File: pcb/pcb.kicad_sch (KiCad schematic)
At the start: 20 parts, among them J1 Conn_01x03_Pin, J2 Screw_Terminal_01x06, J3 Barrel_Jack_Switch, J5 DE9_Plug, U1 74LS165, U2 LM7805_TO220

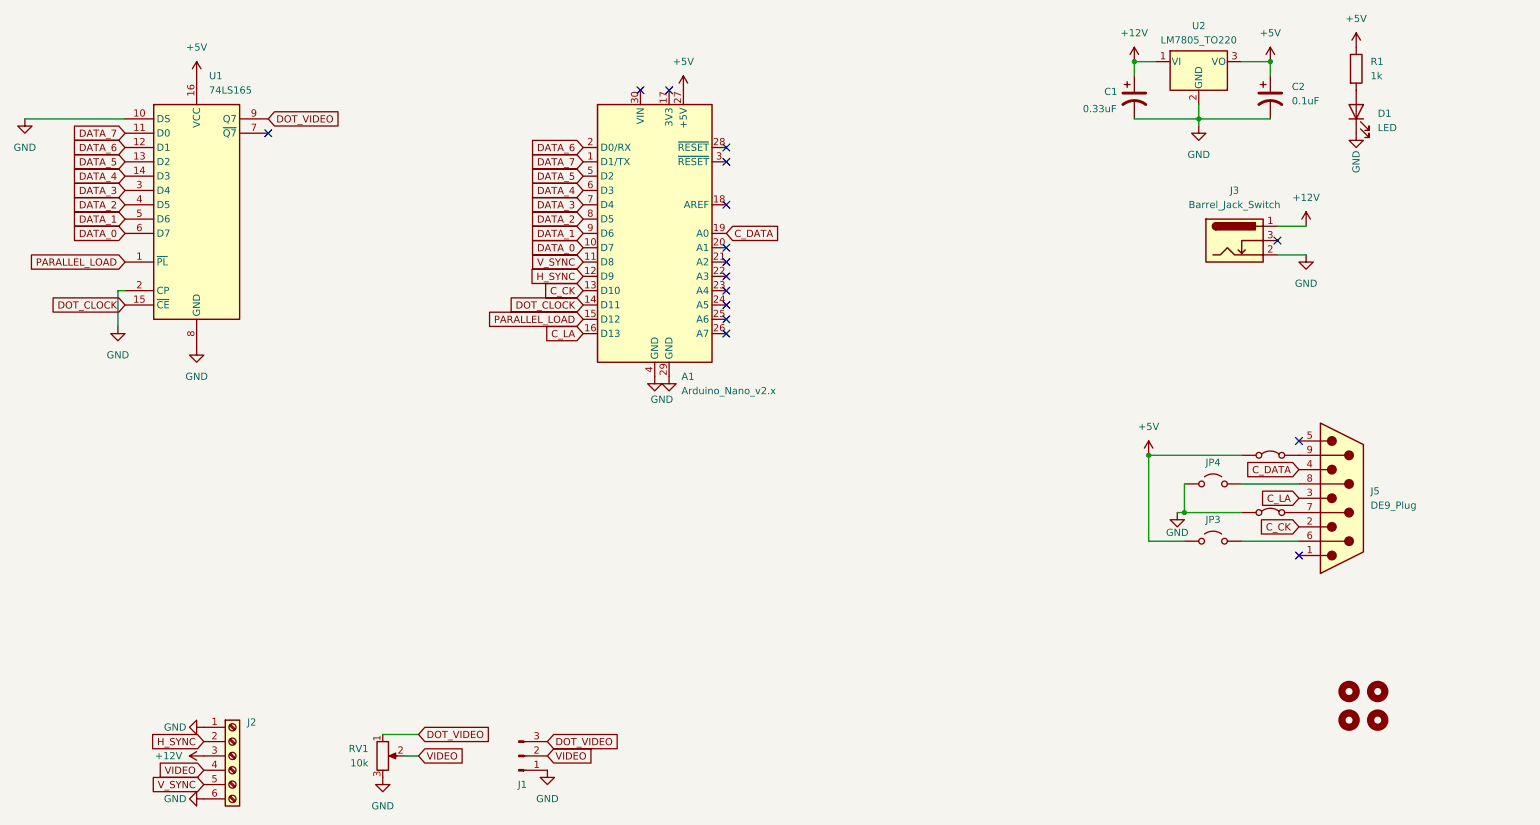
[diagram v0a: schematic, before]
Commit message: New PDB files
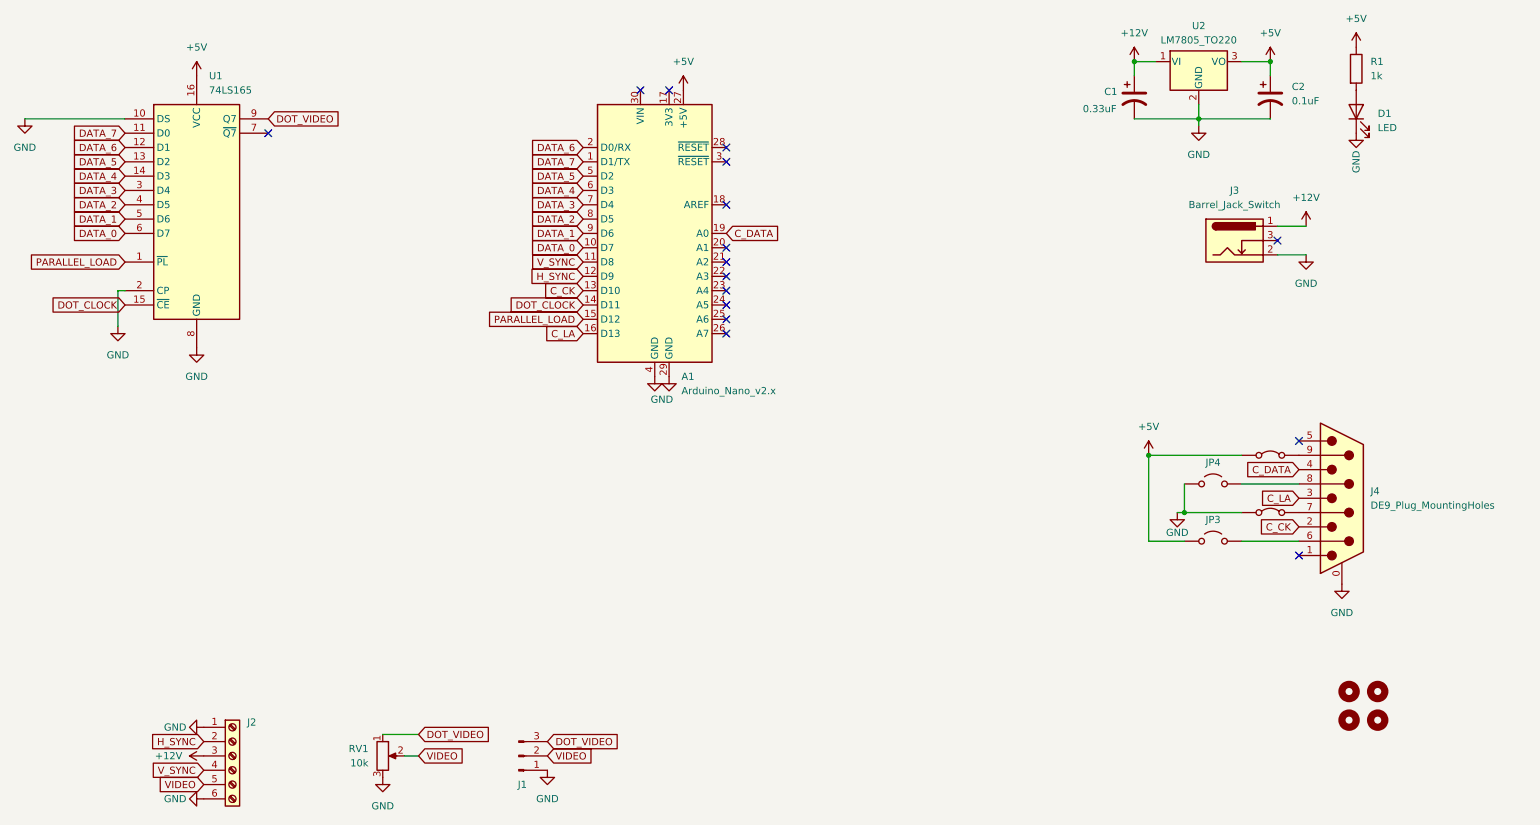
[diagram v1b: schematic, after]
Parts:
- removed J5: DE9_Plug, Connector_Dsub:DSUB-9_Female_Horizontal_P2.77x2.84mm_EdgePinOffset7.70mm_Housed_MountingHolesOffset9.12mm, symbol Connector:DE9_Plug
- added J4: DE9_Plug_MountingHoles, Connector_Dsub:DSUB-9_Female_Horizontal_P2.77x2.84mm_EdgePinOffset7.70mm_Housed_MountingHolesOffset9.12mm, symbol Connector:DE9_Plug_MountingHoles
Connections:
- net C_CK: now also J4.2
- net C_DATA: now also J4.4
- net C_LA: now also J4.3
- net GND: now also J4.0 (PAD)
- net VIDEO: now also J2.5 (Pin_5); no longer J2.4 (Pin_4)
- net V_SYNC: now also J2.4 (Pin_4); no longer J2.5 (Pin_5)
- net at JP3.2 (B): now also J4.6
- net at JP2.2 (B): now also J4.7
- net at JP4.2 (B): now also J4.8
- net at JP1.2 (B): now also J4.9
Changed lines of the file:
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@@
 	(global_label "V_SYNC"
 		(shape input)
-		(at 60.96 161.29 180)
+		(at 60.96 158.75 180)
 		(fields_autoplaced yes)
 		(effects
@@
 		)
 		(property "Intersheetrefs" "${INTERSHEET_REFS}"
-			(at 51.02 161.29 0)
+			(at 51.02 158.75 0)
 			(effects
 				(font
@@
 	(global_label "VIDEO"
 		(shape input)
-		(at 60.96 158.75 180)
+		(at 60.96 161.29 180)
 		(fields_autoplaced yes)
 		(effects
@@
 		)
 		(property "Intersheetrefs" "${INTERSHEET_REFS}"
-			(at 52.5319 158.75 0)
+			(at 52.5319 161.29 0)
 			(effects
 				(font
@@
 	)
 	(symbol
-		(lib_id "Connector:DE9_Plug")
-		(at 262.89 110.49 0)
-		(unit 1)
-		(exclude_from_sim no)
-		(in_bom yes)
-		(on_board yes)
-		(dnp no)
-		(fields_autoplaced yes)
-		(property "Reference" "J5"
-			(at 267.97 109.2199 0)
-			(effects
-				(font
-					(size 1.27 1.27)
-				)
-				(justify left)
-			)
-		)
-		(property "Value" "DE9_Plug"
-			(at 267.97 111.7599 0)
-			(effects
-				(font
-					(size 1.27 1.27)
-				)
-				(justify left)
-			)
-		)
-		(property "Footprint" "Connector_Dsub:DSUB-9_Female_Horizontal_P2.77x2.84mm_EdgePinOffset7.70mm_Housed_MountingHolesOffset9.12mm"
-			(at 262.89 110.49 0)
-			(effects
-				(font
-					(size 1.27 1.27)
-				)
-				(hide yes)
-			)
-		)
-		(property "Datasheet" "~"
-			(at 262.89 110.49 0)
-			(effects
-				(font
-					(size 1.27 1.27)
-				)
-				(hide yes)
-			)
-		)
-		(property "Description" "9-pin male plug pin D-SUB connector"
-			(at 262.89 110.49 0)
-			(effects
-				(font
-					(size 1.27 1.27)
-				)
-				(hide yes)
-			)
-		)
-		(pin "8"
-		)
-		(pin "9"
-		)
-		(pin "1"
-		)
-		(pin "3"
-		)
-		(pin "5"
-		)
-		(pin "7"
-		)
-		(pin "2"
-		)
-		(pin "4"
-		)
-		(pin "6"
-		)
-		(instances
-			(project ""
-				(path "/e222e52e-83a8-4556-a94e-a22482ba41c4"
-					(reference "J5")
-					(unit 1)
-				)
-			)
-		)
-	)
-	(symbol
 		(lib_id "power:GND")
 		(at 233.68 113.03 0)
@@
 	)
 	(symbol
+		(lib_id "Connector:DE9_Plug_MountingHoles")
+		(at 262.89 110.49 0)
+		(unit 1)
+		(exclude_from_sim no)
+		(in_bom yes)
+		(on_board yes)
+		(dnp no)
+		(fields_autoplaced yes)
+		(property "Reference" "J4"
+			(at 267.97 109.2199 0)
+			(effects
+				(font
+					(size 1.27 1.27)
+				)
+				(justify left)
+			)
+		)
+		(property "Value" "DE9_Plug_MountingHoles"
+			(at 267.97 111.7599 0)
+			(effects
+				(font
+					(size 1.27 1.27)
+				)
+				(justify left)
+			)
+		)
+		(property "Footprint" "Connector_Dsub:DSUB-9_Female_Horizontal_P2.77x2.84mm_EdgePinOffset7.70mm_Housed_MountingHolesOffset9.12mm"
+			(at 262.89 110.49 0)
+			(effects
+				(font
+					(size 1.27 1.27)
+				)
+				(hide yes)
+			)
+		)
+		(property "Datasheet" "~"
+			(at 262.89 110.49 0)
+			(effects
+				(font
+					(size 1.27 1.27)
+				)
+				(hide yes)
+			)
+		)
+		(property "Description" "9-pin male plug pin D-SUB connector, Mounting Hole"
+			(at 262.89 110.49 0)
+			(effects
+				(font
+					(size 1.27 1.27)
+				)
+				(hide yes)
+			)
+		)
+		(pin "8"
+		)
+		(pin "0"
+		)
+		(pin "9"
+		)
+		(pin "4"
+		)
+		(pin "6"
+		)
+		(pin "7"
+		)
+		(pin "3"
+		)
+		(pin "5"
+		)
+		(pin "1"
+		)
+		(pin "2"
+		)
+		(instances
+			(project ""
+				(path "/e222e52e-83a8-4556-a94e-a22482ba41c4"
+					(reference "J4")
+					(unit 1)
+				)
+			)
+		)
+	)
+	(symbol
 		(lib_id "power:GND")
 		(at 45.72 80.01 0)
@@
 					(unit 1)
 				)
+			)
+		)
+	)
+	(symbol
+		(lib_id "power:GND")
+		(at 262.89 125.73 0)
+		(unit 1)
+		(exclude_from_sim no)
+		(in_bom yes)
+		(on_board yes)
+		(dnp no)
+		(fields_autoplaced yes)
+		(property "Reference" "#PWR022"
+			(at 262.89 132.08 0)
+			(effects
+				(font
+					(size 1.27 1.27)
+				)
+				(hide yes)
+			)
+		)
+		(property "Value" "GND"
+			(at 262.89 130.81 0)
+			(effects
+				(font
+					(size 1.27 1.27)
+				)
+			)
+		)
+		(property "Footprint" ""
+			(at 262.89 125.73 0)
+			(effects
+				(font
+					(size 1.27 1.27)
+				)
+				(hide yes)
+			)
+		)
+		(property "Datasheet" ""
+			(at 262.89 125.73 0)
+			(effects
+				(font
+					(size 1.27 1.27)
+				)
+				(hide yes)
+			)
+		)
+		(property "Description" "Power symbol creates a global label with name \"GND\" , ground"
+			(at 262.89 125.73 0)
+			(effects
+				(font
+					(size 1.27 1.27)
+				)
+				(hide yes)
+			)
+		)
+		(pin "1"
+		)
+		(instances
+			(project "pcb"
+				(path "/e222e52e-83a8-4556-a94e-a22482ba41c4"
+					(reference "#PWR022")
+					(unit 1)
+				)
